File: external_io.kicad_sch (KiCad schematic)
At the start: 10 parts, among them J1 UJ20-C-H-G-SMT-1-P16-TR, J2 Conn_01x04_Socket, J3 Conn_01x02_Socket, J4 Conn_01x02_Socket, J5 Conn_01x07_Socket, J6 Conn_01x03_Pin, U1 USBLC6-2SC6, U2 USBLC6-2SC6

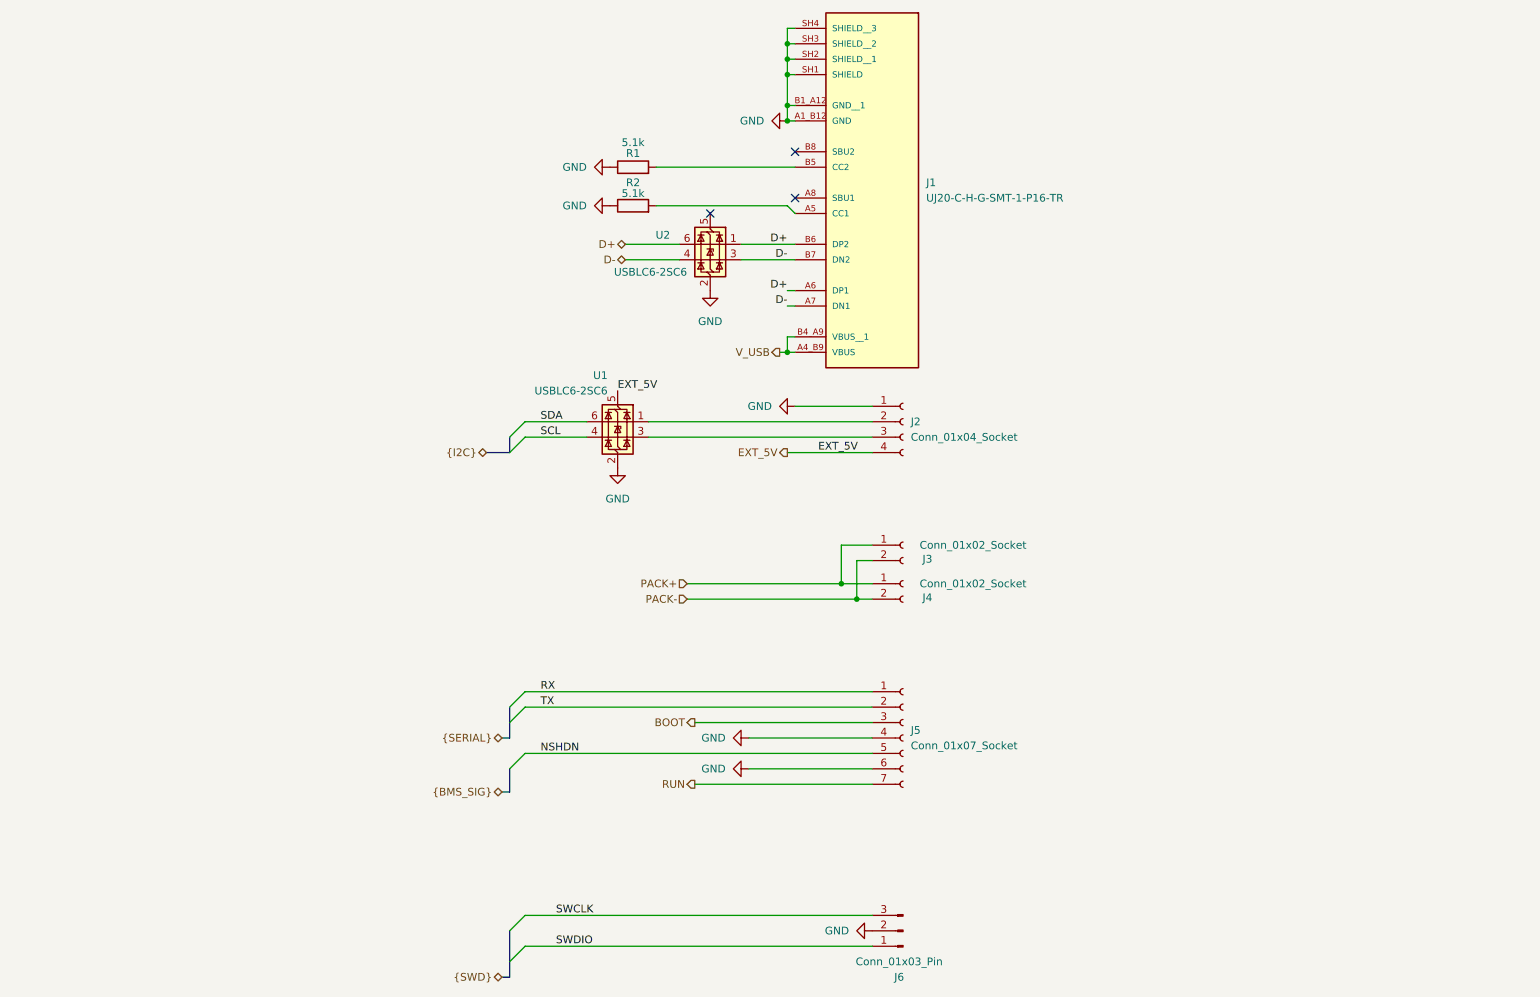
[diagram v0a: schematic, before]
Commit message: Updating stuff
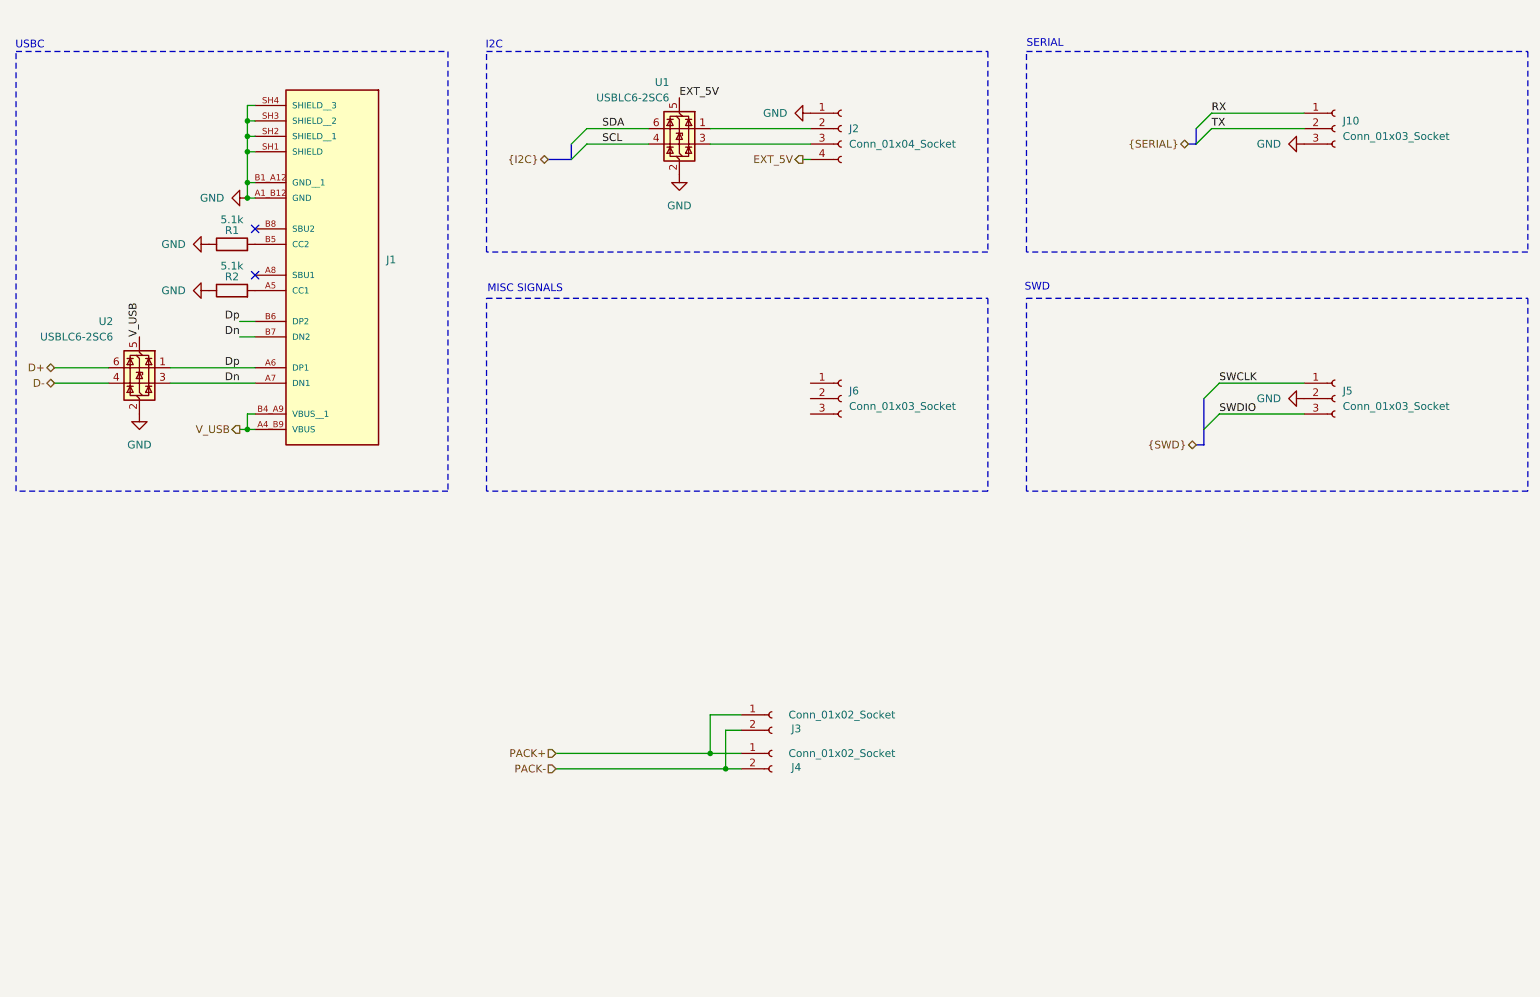
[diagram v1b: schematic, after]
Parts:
- removed J5: Conn_01x07_Socket, Connector_PinHeader_1.00mm:PinHeader_1x07_P1.00mm_Vertical, symbol Connector:Conn_01x07_Socket
- removed J6: Conn_01x03_Pin, Connector_JST:JST_SH_SM03B-SRSS-TB_1x03-1MP_P1.00mm_Horizontal, symbol Connector:Conn_01x03_Pin
- added J10, J5, J6: Conn_01x03_Socket, Connector_PinHeader_2.54mm:PinHeader_1x03_P2.54mm_Vertical, symbol Connector:Conn_01x03_Socket
- R1, R2: Supplier_2 (none) -> JLCPCB; Supplier_2 P/N (none) -> C125891; Supplier_2 Price @ Qty (none) -> 1; Supplier_2 Unit Price (none) -> 0.0024
- U1, U2: Supplier_2 (none) -> JLCPCB; Supplier_2 P/N (none) -> C7519; Supplier_2 Price @ Qty (none) -> 1; Supplier_2 Unit Price (none) -> 0.1373
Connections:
- net D+: no longer J1.A6 (DP1), J1.B6 (DP2), U2.1 (I/O1)
- net D-: no longer J1.A7 (DN1), J1.B7 (DN2), U2.3 (I/O2)
- net GND: now also J10.3 (Pin_3), J5.2 (Pin_2)
- net RX: now also J10.1 (Pin_1)
- net SWCLK: now also J5.1 (Pin_1)
- net SWDIO: now also J5.3 (Pin_3)
- net TX: now also J10.2 (Pin_2)
- net V_USB: now also U2.5 (VBUS)
- new net Dn: J1.A7 (DN1), J1.B7 (DN2), U2.3 (I/O2)
- new net Dp: J1.A6 (DP1), J1.B6 (DP2), U2.1 (I/O1)
- no-connect marks 3 -> 2
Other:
- note added: "I2C"
- note added: "MISC SIGNALS"
- note added: "SERIAL"
- note added: "SWD"
- note added: "USBC"
- moved on the sheet: J1, J2, J3, J4, R1, U1
